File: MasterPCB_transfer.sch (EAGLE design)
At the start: 1070 parts, among them IC1 NCS21911SN2T1G, IC10 LDL1117S33R, IC11 LTC4222CUH#PBF, IC12 LTC4222CUH#PBF, IC13 LTC4222CUH#PBF, IC14 LTC4222CUH#PBF, IC15 LTC4222CUH#PBF, IC16 LTC4222CUH#PBF, IC17 LTC4222CUH#PBF, IC18 LTC4222CUH#PBF, IC19 LTC4222CUH#PBF, IC2 NCS21911SN2T1G, IC20 LTC4222CUH#PBF, IC21 LTC4222CUH#PBF, IC22 LTC4222CUH#PBF, IC23 LTC4222CUH#PBF, IC24 NCS21911SN2T1G, IC25 NCS21911SN2T1G, IC26 NCS21911SN2T1G, IC27 NCS21911SN2T1G, IC28 NCS21911SN2T1G, IC29 NCS21911SN2T1G, IC3 NCS21911SN2T1G, IC30 NCS21911SN2T1G, IC31 ADIS16500AMLZ, IC32 LTC6820IUD#PBF, IC33 CBTL01023GM,115, IC34 MAX889TESA+, IC35 NCS21911SN2T1G, IC36 NCS21911SN2T1G, IC37 NCS21911SN2T1G, IC38 ADS8588HIPM, IC39 NCS21911SN2T1G, IC4 LTC4222CUH#PBF, IC40 NCS21911SN2T1G, IC41 NCS21911SN2T1G, IC42 NCS21911SN2T1G, IC43 NCS21911SN2T1G, IC44 NCS21911SN2T1G, IC45 NCS21911SN2T1G, IC46 NCS21911SN2T1G, IC47 NCS21911SN2T1G, IC48 NCS21911SN2T1G, IC49 NCS21911SN2T1G, IC5 LP38692SDX-5.0_NOPB, IC50 NCS21911SN2T1G, IC51 ADS8588HIPM, IC52 ADS8588HIPM, IC53 NCS21911SN2T1G, IC54 NCS21911SN2T1G, IC55 NCS21911SN2T1G, IC56 NCS21911SN2T1G, IC57 NCS21911SN2T1G, IC58 NCS21911SN2T1G, IC59 NCS21911SN2T1G, IC6 LP38692SDX-5.0_NOPB, IC60 NCS21911SN2T1G, IC61 NCS21911SN2T1G, IC62 NCS21911SN2T1G, IC63 NCS21911SN2T1G, IC64 NCS21911SN2T1G, IC65 NCS21911SN2T1G, IC66 NCS21911SN2T1G, IC67 NCS21911SN2T1G, IC68 NCS21911SN2T1G, IC69 NCS21911SN2T1G, IC7 LDL1117S33R, IC70 NCS21911SN2T1G, IC71 NCS21911SN2T1G, IC72 NCS21911SN2T1G, IC73 NCS21911SN2T1G, IC74 NCS21911SN2T1G, IC75 NCS21911SN2T1G, IC76 NCS21911SN2T1G, IC77 NCS21911SN2T1G, IC78 NCS21911SN2T1G, IC79 NCS21911SN2T1G, IC8 LDL1117S33R, IC9 LP38692SDX-5.0_NOPB, J1 SAMTEC-SMM-104-02-X-DJ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

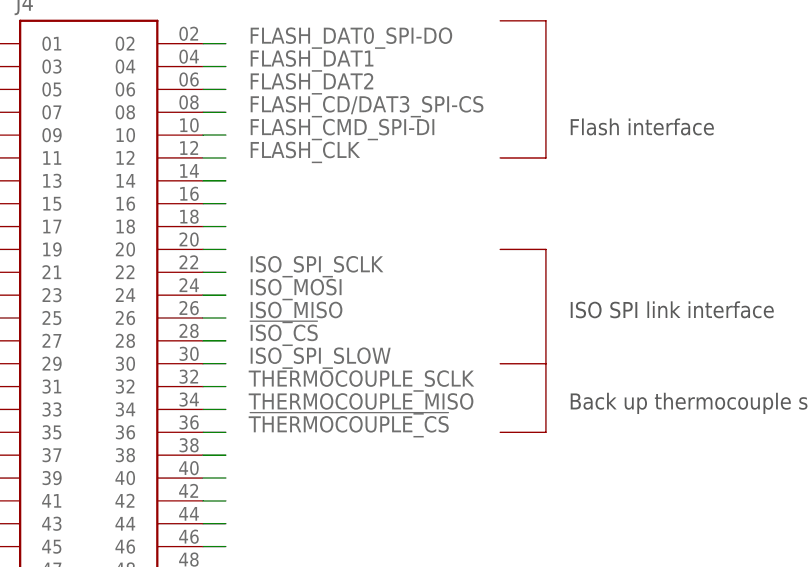
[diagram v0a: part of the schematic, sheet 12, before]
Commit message: Save point
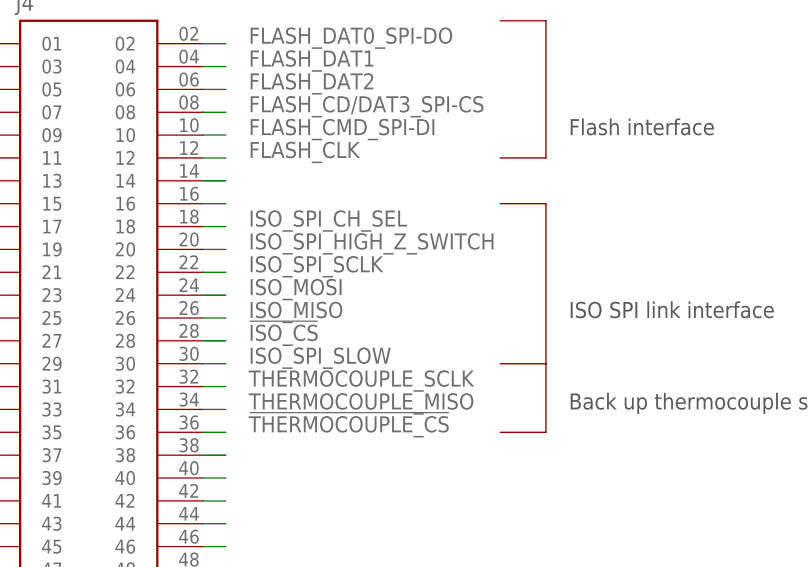
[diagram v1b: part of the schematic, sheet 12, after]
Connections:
- removed net N$43: J4.18
- removed net N$46: J4.20
- net ISO_SPI_CH_SEL: now also J4.18
- net ISO_SPI_HIGH_Z_SWITCH: now also J4.20
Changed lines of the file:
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@@
 <wire x1="236.22" y1="-17.78" x2="241.3" y2="-17.78" width="0.1524" layer="94"/>
 <wire x1="241.3" y1="-17.78" x2="241.3" y2="-33.02" width="0.1524" layer="94"/>
-<wire x1="241.3" y1="-43.18" x2="236.22" y2="-43.18" width="0.1524" layer="94"/>
+<wire x1="241.3" y1="-38.1" x2="236.22" y2="-38.1" width="0.1524" layer="94"/>
 <text x="243.84" y="-30.48" size="1.778" layer="97">Flash interface</text>
-<wire x1="241.3" y1="-43.18" x2="241.3" y2="-55.88" width="0.1524" layer="94"/>
+<wire x1="241.3" y1="-38.1" x2="241.3" y2="-55.88" width="0.1524" layer="94"/>
 <wire x1="241.3" y1="-55.88" x2="236.22" y2="-55.88" width="0.1524" layer="94"/>
 <text x="243.84" y="-50.8" size="1.778" layer="97">ISO SPI link interface</text>
@@
 </segment>
 </net>
-<net name="N$43" class="0">
+<net name="ISO_SPI_CH_SEL" class="0">
 <segment>
 <pinref part="J4" gate="G$1" pin="18"/>
 <wire x1="205.74" y1="-40.64" x2="203.2" y2="-40.64" width="0.1524" layer="91"/>
-</segment>
-</net>
-<net name="N$46" class="0">
+<label x="208.28" y="-40.64" size="1.778" layer="95"/>
+</segment>
+</net>
+<net name="ISO_SPI_HIGH_Z_SWITCH" class="0">
 <segment>
 <pinref part="J4" gate="G$1" pin="20"/>
 <wire x1="205.74" y1="-43.18" x2="203.2" y2="-43.18" width="0.1524" layer="91"/>
-</segment>
-</net>
+<label x="208.28" y="-43.18" size="1.778" layer="95"/>
+</segment>
+</net>
